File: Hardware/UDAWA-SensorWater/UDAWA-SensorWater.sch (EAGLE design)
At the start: 9 parts

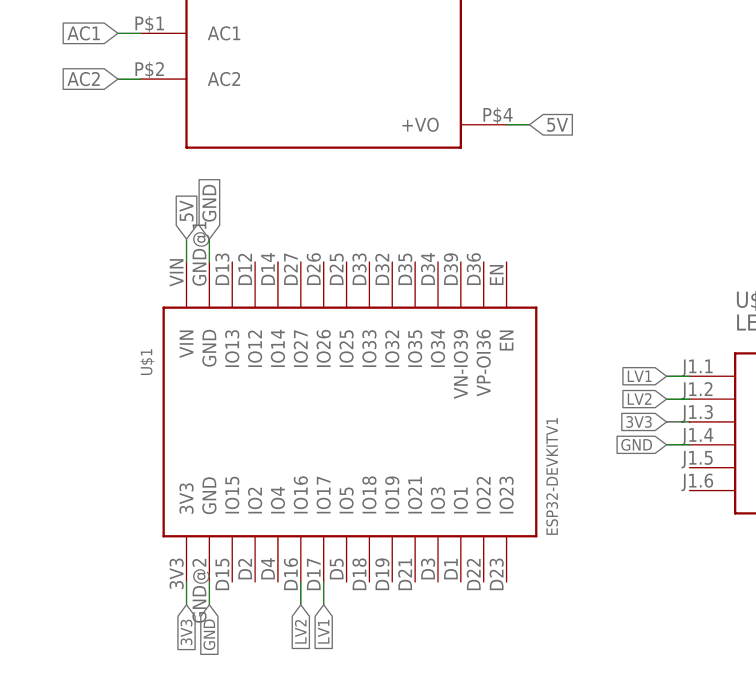
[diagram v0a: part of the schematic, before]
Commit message: Routing PCB #6
Routing PCB
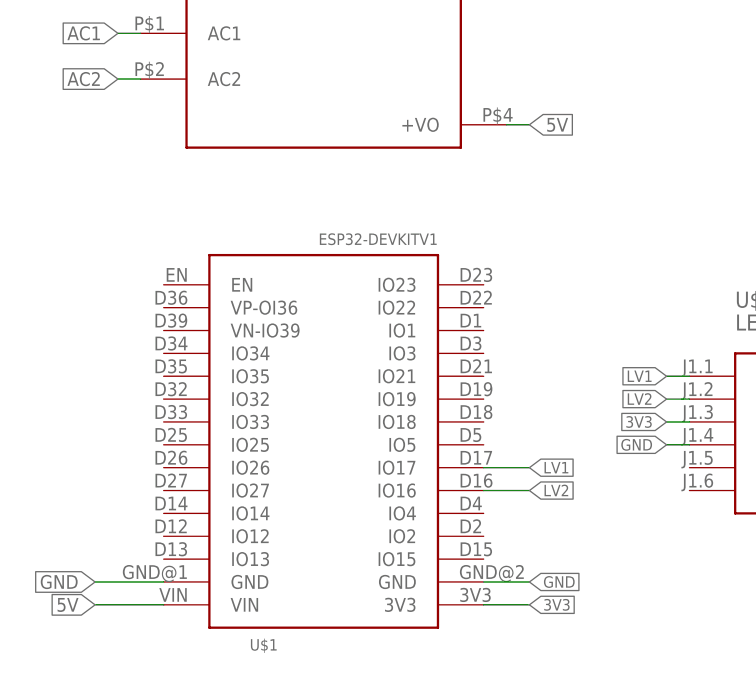
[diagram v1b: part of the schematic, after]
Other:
- moved on the sheet: U$1
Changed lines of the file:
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@@
 </plain>
 <instances>
-<instance part="U$1" gate="G$1" x="-127" y="-35.56" smashed="yes">
-<attribute name="NAME" x="-153.67" y="-30.48" size="1.27" layer="95" rot="R90"/>
+<instance part="U$1" gate="G$1" x="-134.62" y="-33.02" smashed="yes" rot="R90">
+<attribute name="NAME" x="-139.7" y="-59.69" size="1.27" layer="95" rot="R180"/>
 </instance>
 <instance part="HLK1" gate="G$1" x="-134.62" y="5.08" smashed="yes">
@@
 <segment>
 <pinref part="U$1" gate="G$1" pin="GND@1"/>
-<wire x1="-147.32" y1="-17.78" x2="-147.32" y2="-15.24" width="0.1524" layer="91"/>
-<label x="-147.32" y="-15.24" size="1.524" layer="95" rot="R90" xref="yes"/>
+<wire x1="-152.4" y1="-53.34" x2="-160.02" y2="-53.34" width="0.1524" layer="91"/>
+<label x="-160.02" y="-53.34" size="1.524" layer="95" rot="R180" xref="yes"/>
 </segment>
 <segment>
 <pinref part="U$1" gate="G$1" pin="GND@2"/>
-<wire x1="-147.32" y1="-53.34" x2="-147.32" y2="-55.88" width="0.1524" layer="91"/>
-<label x="-147.32" y="-55.88" size="1.27" layer="95" rot="R270" xref="yes"/>
+<wire x1="-116.84" y1="-53.34" x2="-111.76" y2="-53.34" width="0.1524" layer="91"/>
+<label x="-111.76" y="-53.34" size="1.27" layer="95" xref="yes"/>
 </segment>
 <segment>
@@
 <segment>
 <pinref part="U$1" gate="G$1" pin="VIN"/>
-<wire x1="-149.86" y1="-17.78" x2="-149.86" y2="-15.24" width="0.1524" layer="91"/>
-<label x="-149.86" y="-15.24" size="1.524" layer="95" rot="R90" xref="yes"/>
+<wire x1="-152.4" y1="-55.88" x2="-160.02" y2="-55.88" width="0.1524" layer="91"/>
+<label x="-160.02" y="-55.88" size="1.524" layer="95" rot="R180" xref="yes"/>
 </segment>
 <segment>
@@
 <segment>
 <pinref part="U$1" gate="G$1" pin="IO17"/>
-<wire x1="-134.62" y1="-53.34" x2="-134.62" y2="-55.88" width="0.1524" layer="91"/>
-<label x="-134.62" y="-55.88" size="1.27" layer="95" rot="R270" xref="yes"/>
+<wire x1="-116.84" y1="-40.64" x2="-111.76" y2="-40.64" width="0.1524" layer="91"/>
+<label x="-111.76" y="-40.64" size="1.27" layer="95" xref="yes"/>
 </segment>
 </net>
@@
 <segment>
 <pinref part="U$1" gate="G$1" pin="IO16"/>
-<wire x1="-137.16" y1="-53.34" x2="-137.16" y2="-55.88" width="0.1524" layer="91"/>
-<label x="-137.16" y="-55.88" size="1.27" layer="95" rot="R270" xref="yes"/>
+<wire x1="-116.84" y1="-43.18" x2="-111.76" y2="-43.18" width="0.1524" layer="91"/>
+<label x="-111.76" y="-43.18" size="1.27" layer="95" xref="yes"/>
 </segment>
 </net>
@@
 <segment>
 <pinref part="U$1" gate="G$1" pin="3V3"/>
-<wire x1="-149.86" y1="-53.34" x2="-149.86" y2="-55.88" width="0.1524" layer="91"/>
-<label x="-149.86" y="-55.88" size="1.27" layer="95" rot="R270" xref="yes"/>
+<wire x1="-116.84" y1="-55.88" x2="-111.76" y2="-55.88" width="0.1524" layer="91"/>
+<label x="-111.76" y="-55.88" size="1.27" layer="95" xref="yes"/>
 </segment>
 </net>
